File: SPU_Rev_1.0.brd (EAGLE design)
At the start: 162.6 x 106.9 mm, 176 parts, among them IC1 THN10-2411WIR, IC10 MCP6064-E/SL, IC12 LM78L05ACMX/NOPB, IC13 CH340G, IC2 MCP6064-E/SL, IC3 MCP6064-E/SL, IC4 MCP6064-E/SL, IC5 MAX488CSA, IC6 MOCD207MSOIC-8, IC7 MOCD207MSOIC-8, IC8 MOCD207MSOIC-8, IC9 MCP6064-E/SL, Q1 12MHz, U1 ADR366WAUJZ, U10 ADS1148QPWRQ1, U11 ADS1148QPWRQ1, U12 ADS1148QPWRQ1, U13 ADR366WAUJZ, U2 ADR366WAUJZ, U3 ADS1148QPWRQ1, U4 ADS1148QPWRQ1, U5 ADS1148QPWRQ1, U6 LT1528, U7 S70FL01GS, U8 S70FL01GS, U9 STM32F77XXXLQFP208, X1 D-SUB9-H5M09RA, X2 D-SUB15-H5M15RA, X3 USBPTH

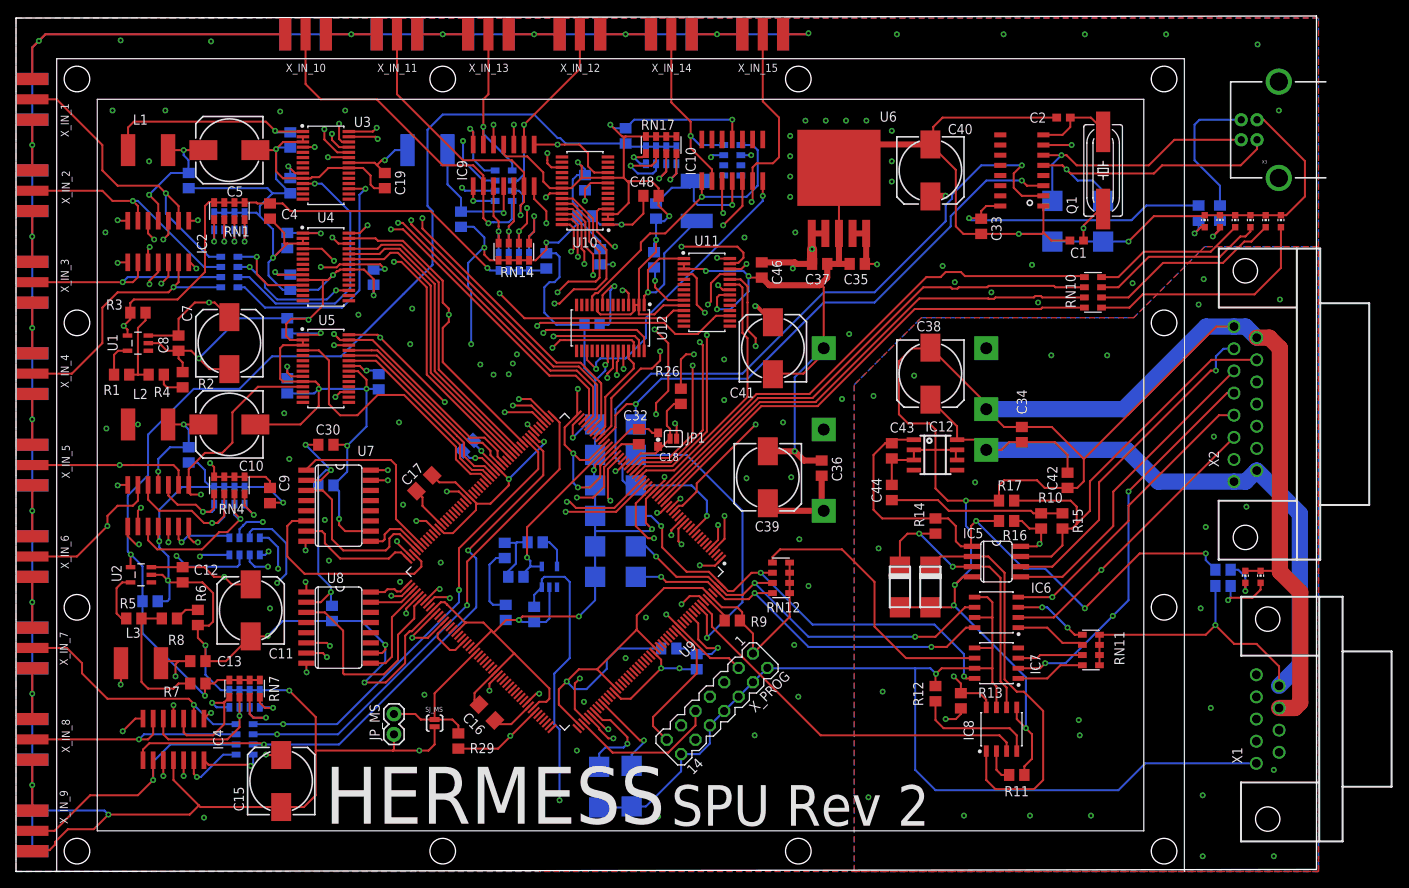
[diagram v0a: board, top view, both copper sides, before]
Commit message: Renamed to SPU_Rev_xx
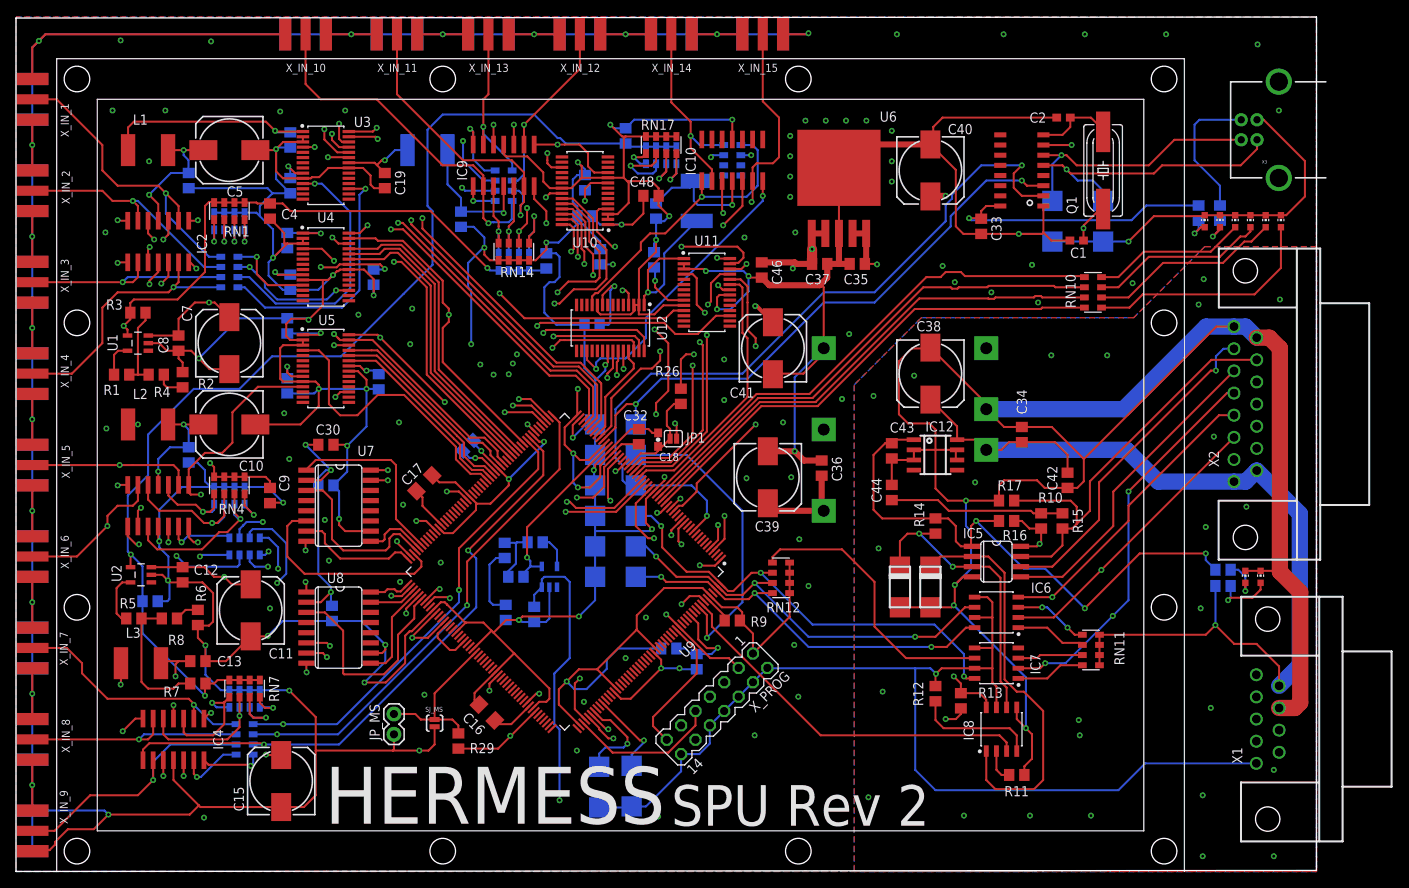
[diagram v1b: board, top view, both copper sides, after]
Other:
- board size 162.6 x 106.9 mm -> 162.6 x 106.8 mm
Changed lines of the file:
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@@
 <layer number="28" name="bValues" color="7" fill="1" visible="no" active="yes"/>
 <layer number="29" name="tStop" color="7" fill="3" visible="no" active="yes"/>
-<layer number="30" name="bStop" color="7" fill="6" visible="no" active="yes"/>
+<layer number="30" name="bStop" color="7" fill="6" visible="yes" active="yes"/>
 <layer number="31" name="tCream" color="7" fill="4" visible="no" active="yes"/>
 <layer number="32" name="bCream" color="7" fill="5" visible="no" active="yes"/>
@@
 <fusionsync huburn="a.cGVyc29uYWw6dWUyYjZiNTFm" projecturn="a.cGVyc29uYWw6dWUyYjZiNTFmIzIwMTcwNjIzODEzNzU4MjY" f3durn="urn:adsk.wipprod:dm.lineage:NfGnPIWBTjK9hH2zAlQcMw" pcbguid="14fbca52-fa02-4b22-b74a-d786bfe443d1" lastpulledtime="" lastsyncedchangeguid="1dbc08e2-01f0-93f9-06e5-93317fdff8ee"/>
 <plain>
-<wire x1="0" y1="0" x2="162.56" y2="0.254" width="0" layer="20"/>
-<wire x1="162.56" y1="0.254" x2="162.56" y2="106.934" width="0" layer="20"/>
-<wire x1="162.56" y1="106.934" x2="0" y2="106.68" width="0" layer="20"/>
+<wire x1="0" y1="0" x2="162.56" y2="0.127" width="0" layer="20"/>
+<wire x1="162.56" y1="0.127" x2="162.56" y2="106.807" width="0" layer="20"/>
+<wire x1="162.56" y1="106.807" x2="0" y2="106.68" width="0" layer="20"/>
 <wire x1="0" y1="106.68" x2="0" y2="0" width="0" layer="20"/>
 <polygon width="0.1524" layer="39">
@@
 <contactref element="IC13" pad="1"/>
 <polygon width="0.3048" layer="1" isolate="0.3048" rank="2">
-<vertex x="0" y="106.68"/>
+<vertex x="0" y="106.807"/>
 <vertex x="0" y="0"/>
-<vertex x="162.814" y="0"/>
-<vertex x="162.814" y="106.68"/>
+<vertex x="162.56" y="0"/>
+<vertex x="162.56" y="106.807"/>
 </polygon>
 <polygon width="0.3048" layer="16" isolate="0.3048" rank="2">
-<vertex x="162.814" y="106.68"/>
-<vertex x="162.814" y="0"/>
+<vertex x="162.56" y="106.807"/>
+<vertex x="162.56" y="0"/>
 <vertex x="0" y="0"/>
-<vertex x="0" y="106.68"/>
+<vertex x="0" y="106.807"/>
 </polygon>
 <contactref element="C1" pad="2"/>
@@
 <wire x1="73.9917" y1="82.165" x2="73.9917" y2="81.515" width="0.254" layer="1"/>
 <polygon width="0.3048" layer="2" isolate="0.3048" rank="2">
-<vertex x="162.814" y="106.68"/>
-<vertex x="162.814" y="0"/>
+<vertex x="162.56" y="106.807"/>
+<vertex x="162.56" y="0"/>
 <vertex x="0" y="0"/>
-<vertex x="0" y="106.68"/>
+<vertex x="0" y="106.807"/>
 </polygon>
 <polygon width="0.3048" layer="15" isolate="0.3048" rank="2">
-<vertex x="162.814" y="106.68"/>
-<vertex x="162.814" y="0"/>
+<vertex x="162.56" y="106.807"/>
+<vertex x="162.56" y="0"/>
 <vertex x="0" y="0"/>
-<vertex x="0" y="106.68"/>
+<vertex x="0" y="106.807"/>
 </polygon>
 <via x="56.896" y="65.913" extent="1-16" drill="0.35"/>
@@
 <contactref element="LED8" pad="C"/>
 <polygon width="0.3048" layer="1" isolate="0.6096">
-<vertex x="162.814" y="78.105"/>
+<vertex x="162.56" y="78.105"/>
 <vertex x="148.59" y="78.105"/>
 <vertex x="139.7" y="69.215"/>
@@
 <vertex x="104.775" y="60.833"/>
 <vertex x="104.775" y="0"/>
-<vertex x="162.814" y="0"/>
+<vertex x="162.56" y="0"/>
 </polygon>
 <polygon width="0.3048" layer="16" isolate="0.6096">
@@
 <vertex x="139.7" y="69.215"/>
 <vertex x="148.59" y="78.105"/>
-<vertex x="162.814" y="78.105"/>
-<vertex x="162.814" y="0"/>
+<vertex x="162.56" y="78.105"/>
+<vertex x="162.56" y="0"/>
 <vertex x="104.775" y="0"/>
 <vertex x="104.775" y="60.833"/>
@@
 <vertex x="139.7" y="69.215"/>
 <vertex x="148.59" y="78.105"/>
-<vertex x="162.814" y="78.105"/>
-<vertex x="162.814" y="0"/>
+<vertex x="162.56" y="78.105"/>
+<vertex x="162.56" y="0"/>
 <vertex x="104.775" y="0"/>
 <vertex x="104.775" y="60.833"/>
@@
 <vertex x="139.7" y="69.215"/>
 <vertex x="148.59" y="78.105"/>
-<vertex x="162.814" y="78.105"/>
-<vertex x="162.814" y="0"/>
+<vertex x="162.56" y="78.105"/>
+<vertex x="162.56" y="0"/>
 <vertex x="104.775" y="0"/>
 <vertex x="104.775" y="60.833"/>
